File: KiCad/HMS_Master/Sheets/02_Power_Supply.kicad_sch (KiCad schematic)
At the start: 4 parts, among them Q1 S8050, U19 BUZZER_SOCKET

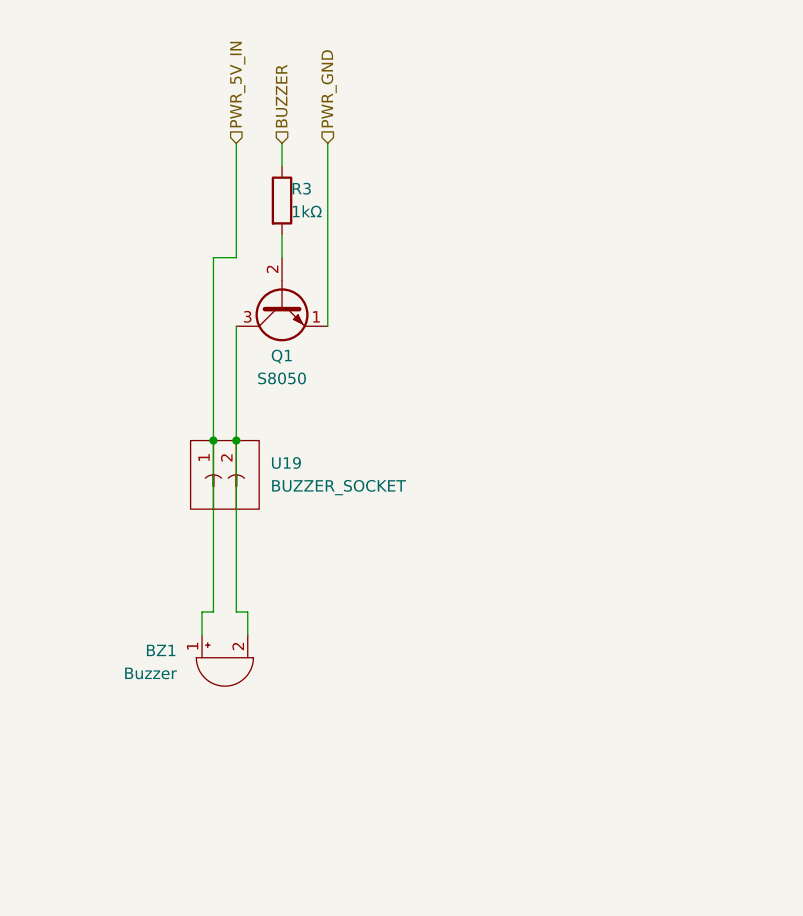
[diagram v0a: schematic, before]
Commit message: Refactor KiCad Master directory structure
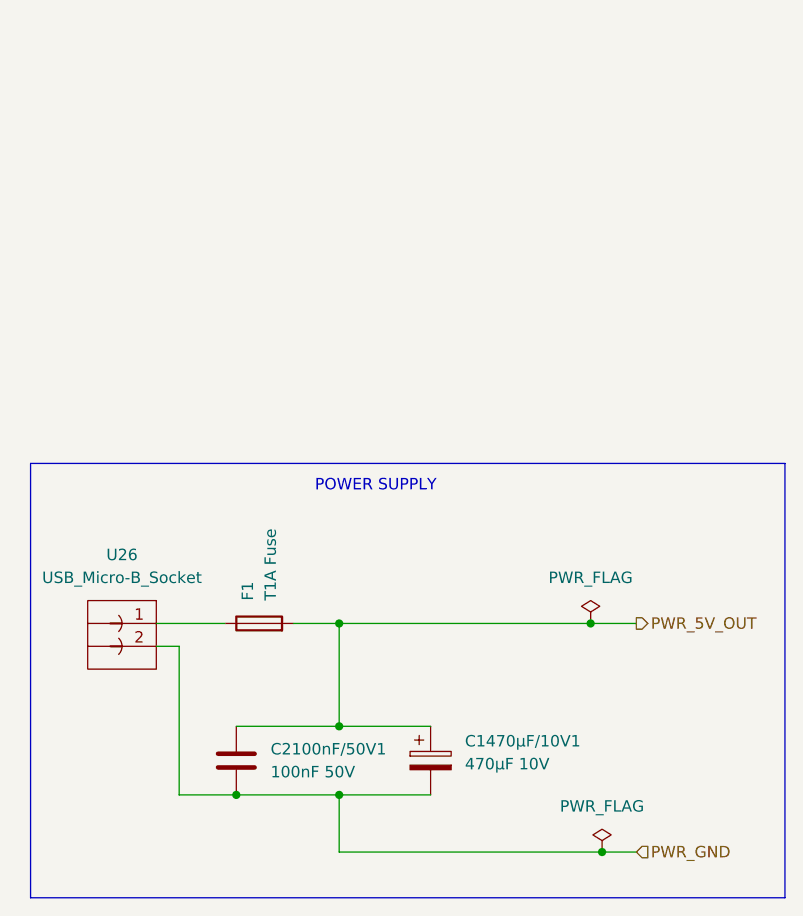
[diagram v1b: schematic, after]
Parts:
- removed BZ1: Buzzer, Buzzer_Beeper:Buzzer_12x9.5RM7.6, symbol Device:Buzzer
- removed Q1: S8050, Package_TO_SOT_THT:TO-92_Inline_Wide, symbol Transistor_BJT:S8050
- removed R3: 1kΩ, Resistor_THT:R_Axial_DIN0207_L6.3mm_D2.5mm_P7.62mm_Horizontal, symbol Device:R
- removed U19: BUZZER_SOCKET, Connector_JST:JST_XH_B2B-XH-A_1x02_P2.50mm_Vertical, symbol HMS_Symbols:CONN_JST_PH_2P
- added C1470µF/10V1: 470µF 10V, Capacitor_THT:CP_Radial_D8.0mm_P3.50mm, symbol Device:C_Polarized
- added C2100nF/50V1: 100nF 50V, Capacitor_THT:C_Disc_D3.8mm_W2.6mm_P2.50mm, symbol Device:C
- added F1: T1A Fuse, Fuse:Fuseholder_Cylinder-5x20mm_Schurter_0031_8201_Horizontal_Open, symbol Device:Fuse
- added U26: USB_Micro-B_Socket, Connector_JST:JST_XH_B2B-XH-A_1x02_P2.50mm_Vertical, symbol HMS_Symbols:CONN_JST_PH_2P
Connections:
- net PWR_GND: now also C1470µF/10V1.2, C2100nF/50V1.2, U26.2
- new net: F1.1, U26.1
- new net PWR_5V_OUT: C1470µF/10V1.1, C2100nF/50V1.1, F1.2
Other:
- note added: "POWER SUPPLY"
- title: (none) -> HMS-Master
